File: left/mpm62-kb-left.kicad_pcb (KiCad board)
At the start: 2 copper layers, 138.1 x 95.2 mm, 68 parts, among them J1 Conn_01x04_Male, J2 Conn_01x02_Male, SW1 SW_Push, U1 ProMicro

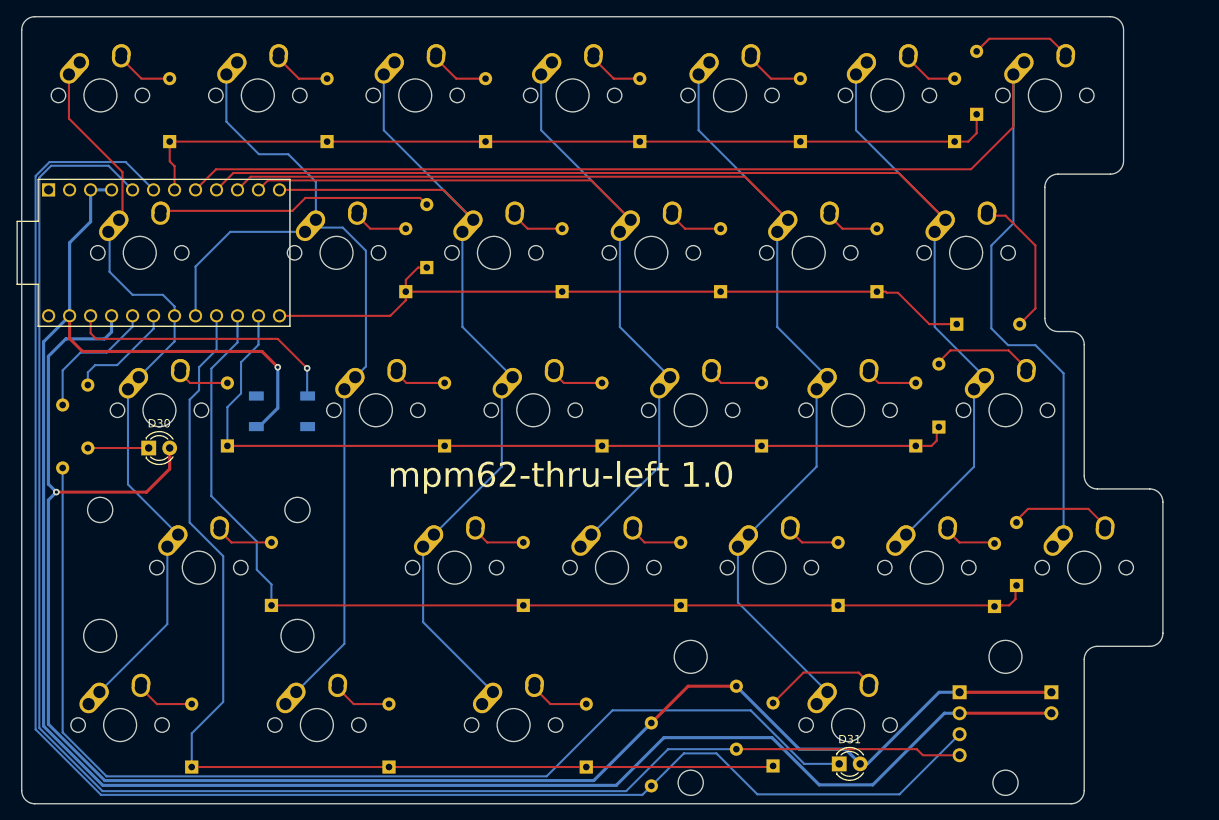
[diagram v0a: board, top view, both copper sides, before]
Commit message: Final for b1t (board 1 thruhole) board
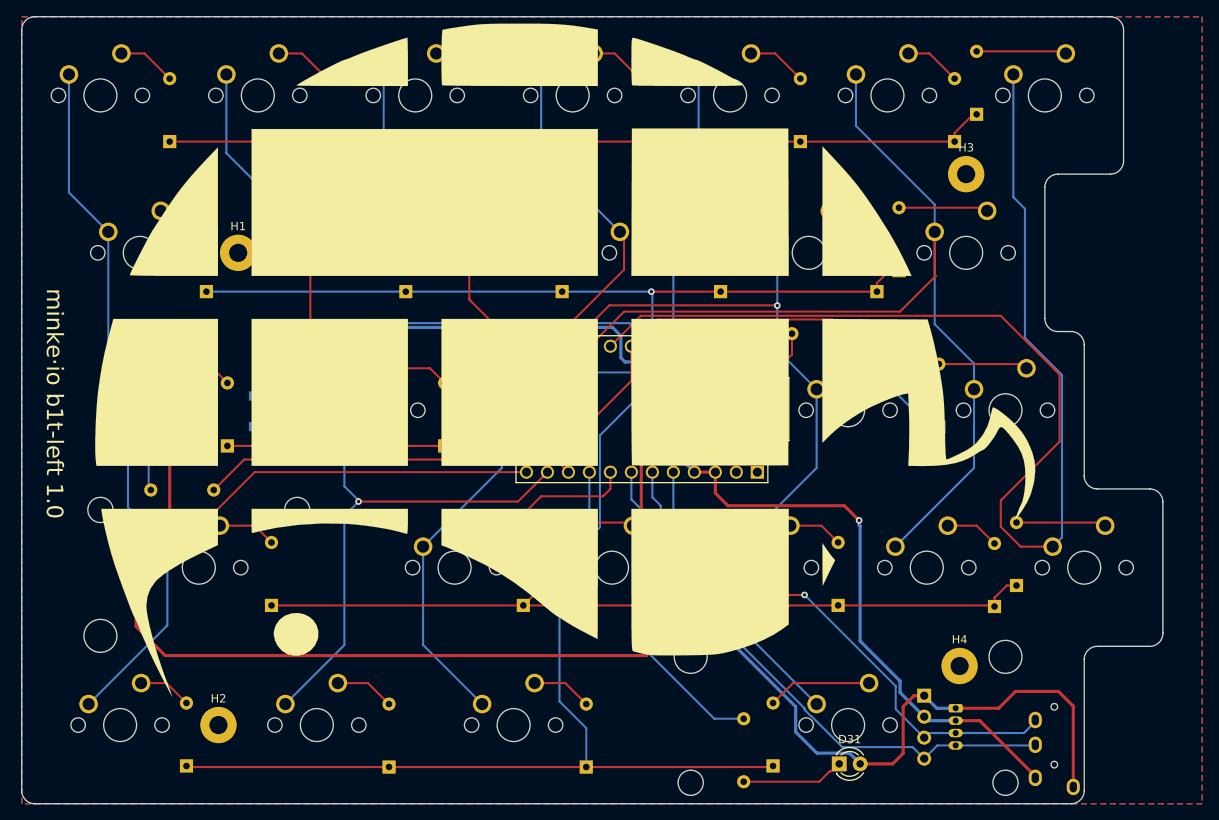
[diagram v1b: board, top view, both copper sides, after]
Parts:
- added G***: LOGO, MpmMisc:small_logo, B.Cu at (121.4, 108.7)
- added G***: LOGO, MpmMisc:biglogo3, F.Cu at (144.4, 73.9)
- added H1: MountingHole, MountingHole:MountingHole_2.2mm_M2_Pad, F.Cu at (105.6, 60.3)
- added H2: MountingHole, MountingHole:MountingHole_2.2mm_M2_Pad, F.Cu at (103.2, 117.5)
- added H3: MountingHole, MountingHole:MountingHole_2.2mm_M2_Pad, F.Cu at (193.7, 50.8)
- added H4: MountingHole, MountingHole:MountingHole_2.2mm_M2_Pad, F.Cu at (192.9, 110.3)
- added U2: TRRS, Keebio-Parts:TRRS-PJ-320A, B.Cu at (204.3, 113.7)
- J1: value Conn_01x04_Male -> Raw Header
- J2: value Conn_01x02_Male -> JST ZH header; footprint Connector_PinHeader_2.54mm:PinHeader_1x02_P2.54mm_Vertical -> MpmMisc:JST_ZH_B4B-ZR_1x04_P1.50mm_Vertical
- MX1, MX10, MX11, MX12, MX13, MX15, MX16, MX17, MX18, MX19, MX20, MX21, MX22, MX24, MX25, MX26, MX27, MX28, MX29, MX6, MX7, MX8: footprint MX_Alps_Hybrid:MX-1U-NoLED -> MX_Only:MXOnly-1U-NoLED
- MX14, MX5, MX9: footprint MX_Alps_Hybrid:MX-1.25U-NoLED -> MX_Only:MXOnly-1.25U-NoLED
- MX2: footprint MX_Alps_Hybrid:MX-1.5U-NoLED -> MX_Only:MXOnly-1.5U-NoLED
- MX23: footprint MX_Alps_Hybrid:MX-3U-ReversedStabilizers-NoLED -> MX_Only:MXOnly-3U-ReversedStabilizers-NoLED
- MX3: footprint MX_Alps_Hybrid:MX-1.75U-NoLED -> MX_Only:MXOnly-1.75U-NoLED
- MX4: footprint MX_Alps_Hybrid:MX-2.25U-NoLED -> MX_Only:MXOnly-2.25U-NoLED
- moved R2 90.7 mm to (166.8, 124.3)
- moved U1 60.8 mm to (154.4, 79.2), turned to 180 degrees
- moved D2 26.8 mm to (101.7, 65.0)
- moved D17 17.7 mm to (180.2, 70.1), turned to 180 degrees
- moved D18 16.7 mm to (142.6, 100.6)
- moved D12 16.5 mm to (133.2, 81.5)
- moved R4 12.6 mm to (158.9, 105.0), turned to 90 degrees
- moved J2 11.7 mm to (192.4, 115.4), turned to 270 degrees
- moved D25 9.53 mm to (185.5, 62.5), turned to 90 degrees
- moved R1 9.16 mm to (95.0, 89.0), turned to 0 degrees
- moved R3 8.69 mm to (161.9, 105.0), turned to 90 degrees
- moved J1 4.31 mm to (188.6, 113.9)
- moved D5 0.65 mm to (99.3, 122.4)
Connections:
- U1 pad 10: COL4 -> Net-(R1-Pad2)
- U1 pad 11: COL3 -> COL1
- U1 pad 12: COL2 -> COL0
- U1 pad 13: ROW1 -> COL2
- U1 pad 14: ROW2 -> COL3
- U1 pad 15: ROW3 -> COL4
- U1 pad 16: ROW4 -> COL5
- U1 pad 17: COL1 -> COL6
- U1 pad 18: COL0 -> ROW2
- U1 pad 19: Net-(R1-Pad2) -> ROW1
- U1 pad 20: Net-(R2-Pad2) -> ROW0
- U1 pad 7: ROW0 -> Net-(R2-Pad2)
- U1 pad 8: COL6 -> ROW3
- U1 pad 9: COL5 -> ROW4
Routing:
- net Net-(J1-Pad3): track 205.6 -> 67.7 mm, vias 0 -> 1
- net Net-(J1-Pad4): track 197.2 -> 66.4 mm
- net Net-(D31-Pad1): track 134.2 -> 12.5 mm
- net GND: track 240.9 -> 158.7 mm
- net COL0: track 88.4 -> 132.3 mm
- net COL4: track 154.7 -> 117.4 mm, vias 0 -> 1
- net COL5: track 154.6 -> 117.8 mm
- net COL3: track 112.7 -> 80.5 mm
- net Net-(R1-Pad2): track 13.2 -> 45.1 mm
- net Net-(D2-Pad2): track 33.5 -> 6.67 mm
- net COL6: track 172.8 -> 147.5 mm
- net Net-(SW1-Pad1): track 33.6 -> 57.9 mm, vias 1 -> 0
- net Net-(R2-Pad2): track 16.2 -> 38.4 mm
- net ROW4: track 129.6 -> 108.9 mm
- net ROW0: track 106.5 -> 126.1 mm
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- added copper zone on B.Cu, net GND
- added copper zone on F.Cu, net GND
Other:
- board text added: "minke·io b1t-left 1.0"
- board text removed: "mpm62-thru-left 1.0"
